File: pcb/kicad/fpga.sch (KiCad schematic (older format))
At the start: 1 part, among them U4 XC3S400-PQ208

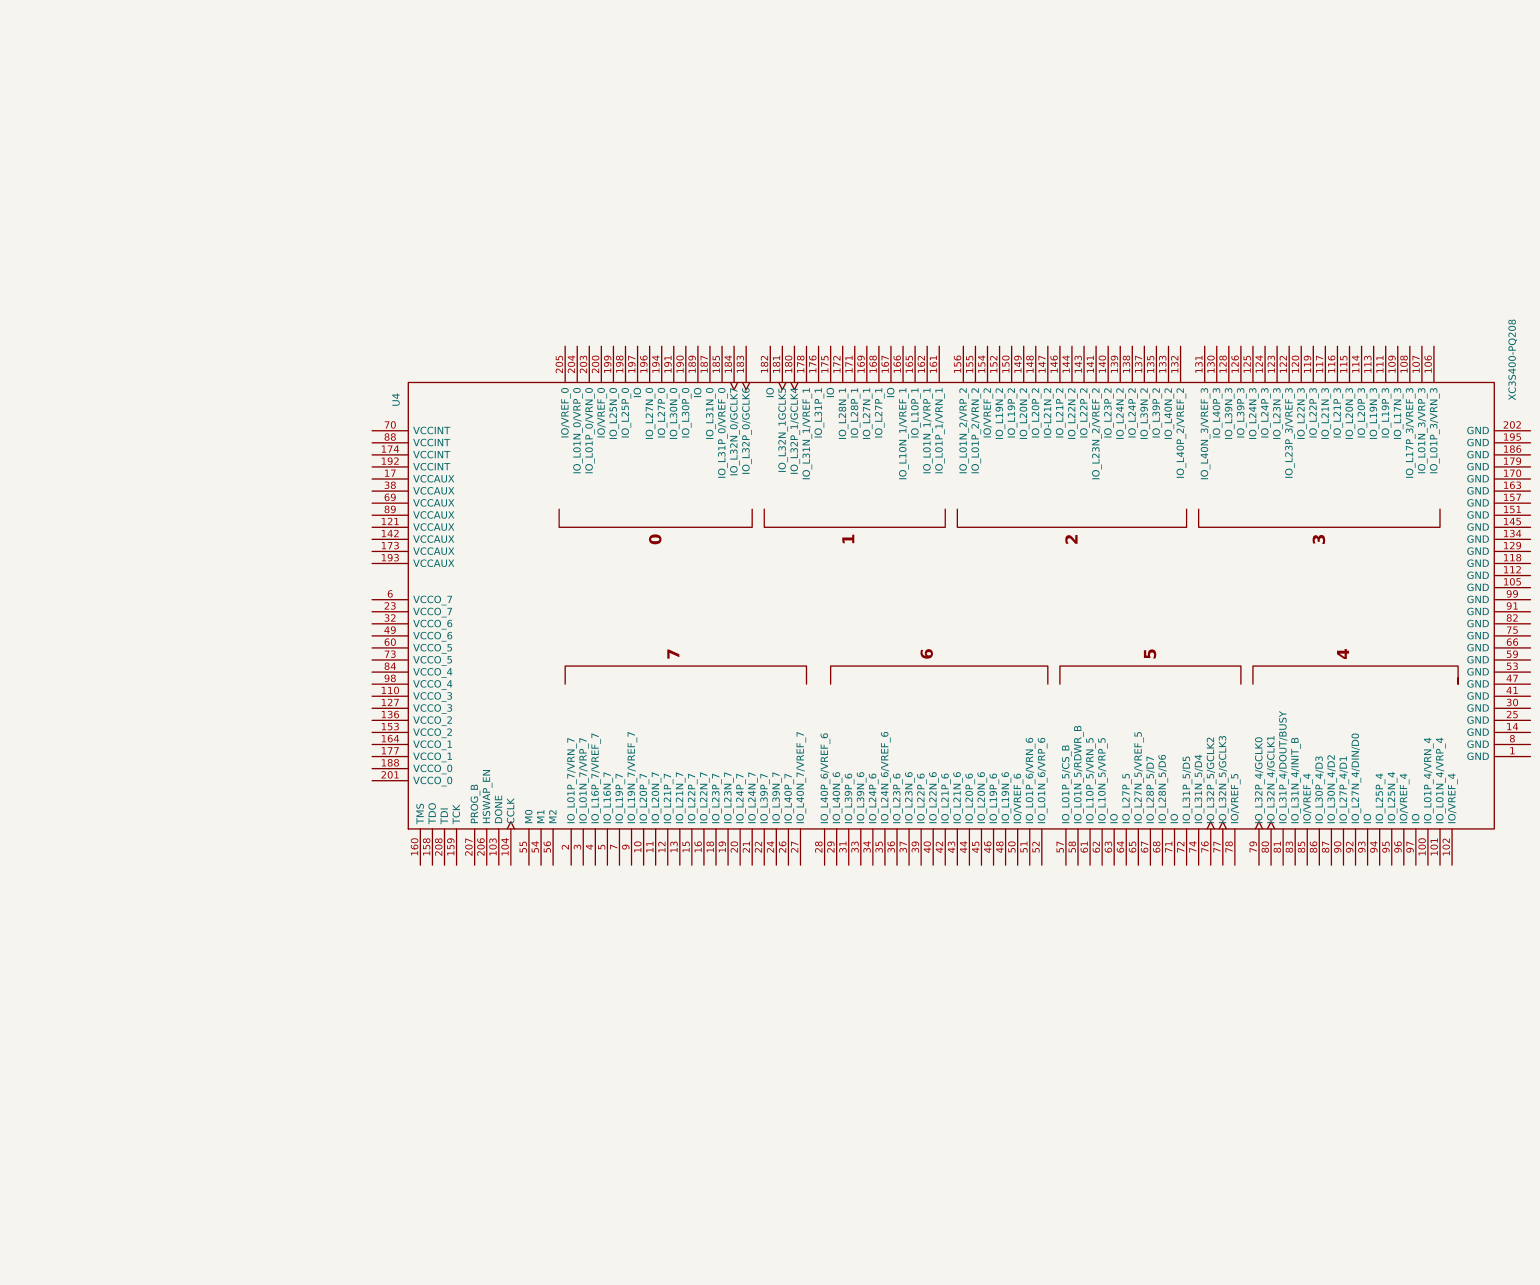
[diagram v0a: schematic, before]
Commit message: kicad wip
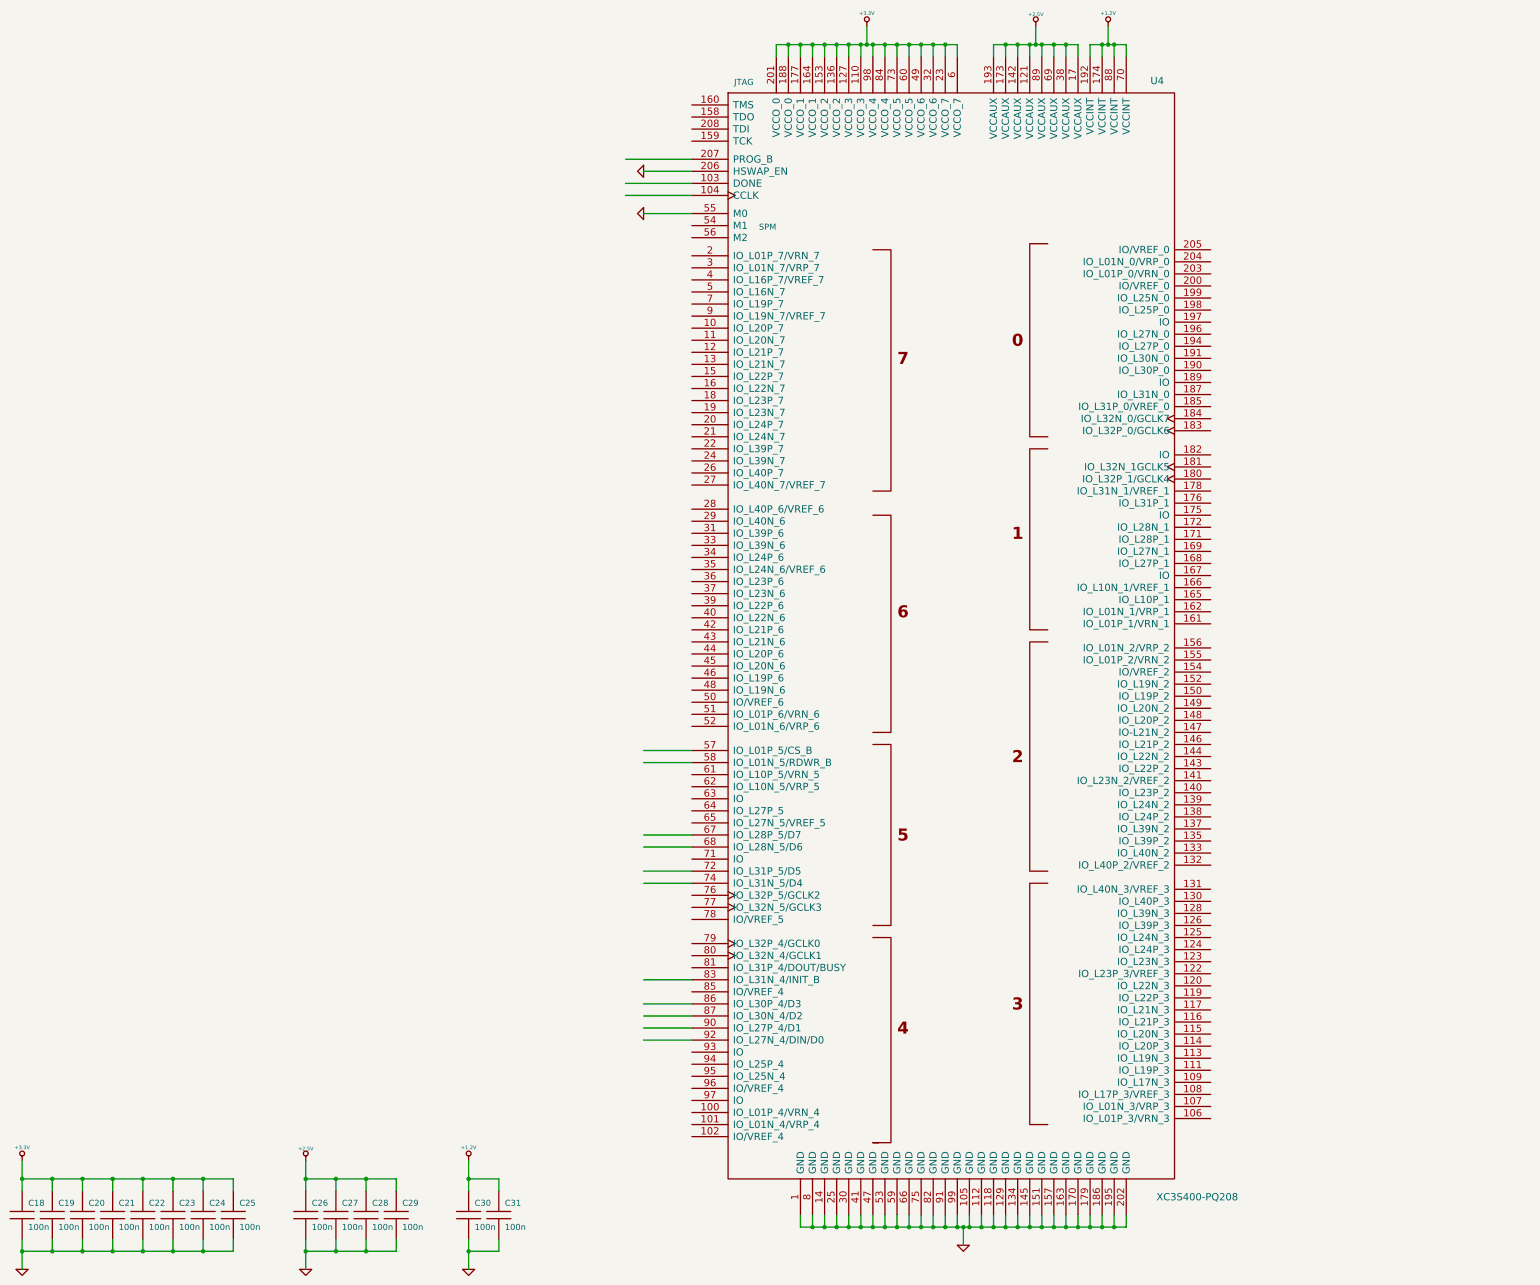
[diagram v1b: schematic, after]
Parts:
- added C18, C19, C20, C21, C22, C23, C24, C25, C26, C27, C28, C29, C30, C31: 100n, symbol C
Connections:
- net labels added: +1.2V, +2.5V, +3.3V, GND
- wire segments 0 -> 114
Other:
- note added: "JTAG"
- note added: "SPM"
- moved on the sheet: U4

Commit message: Schematics+PCB WIP
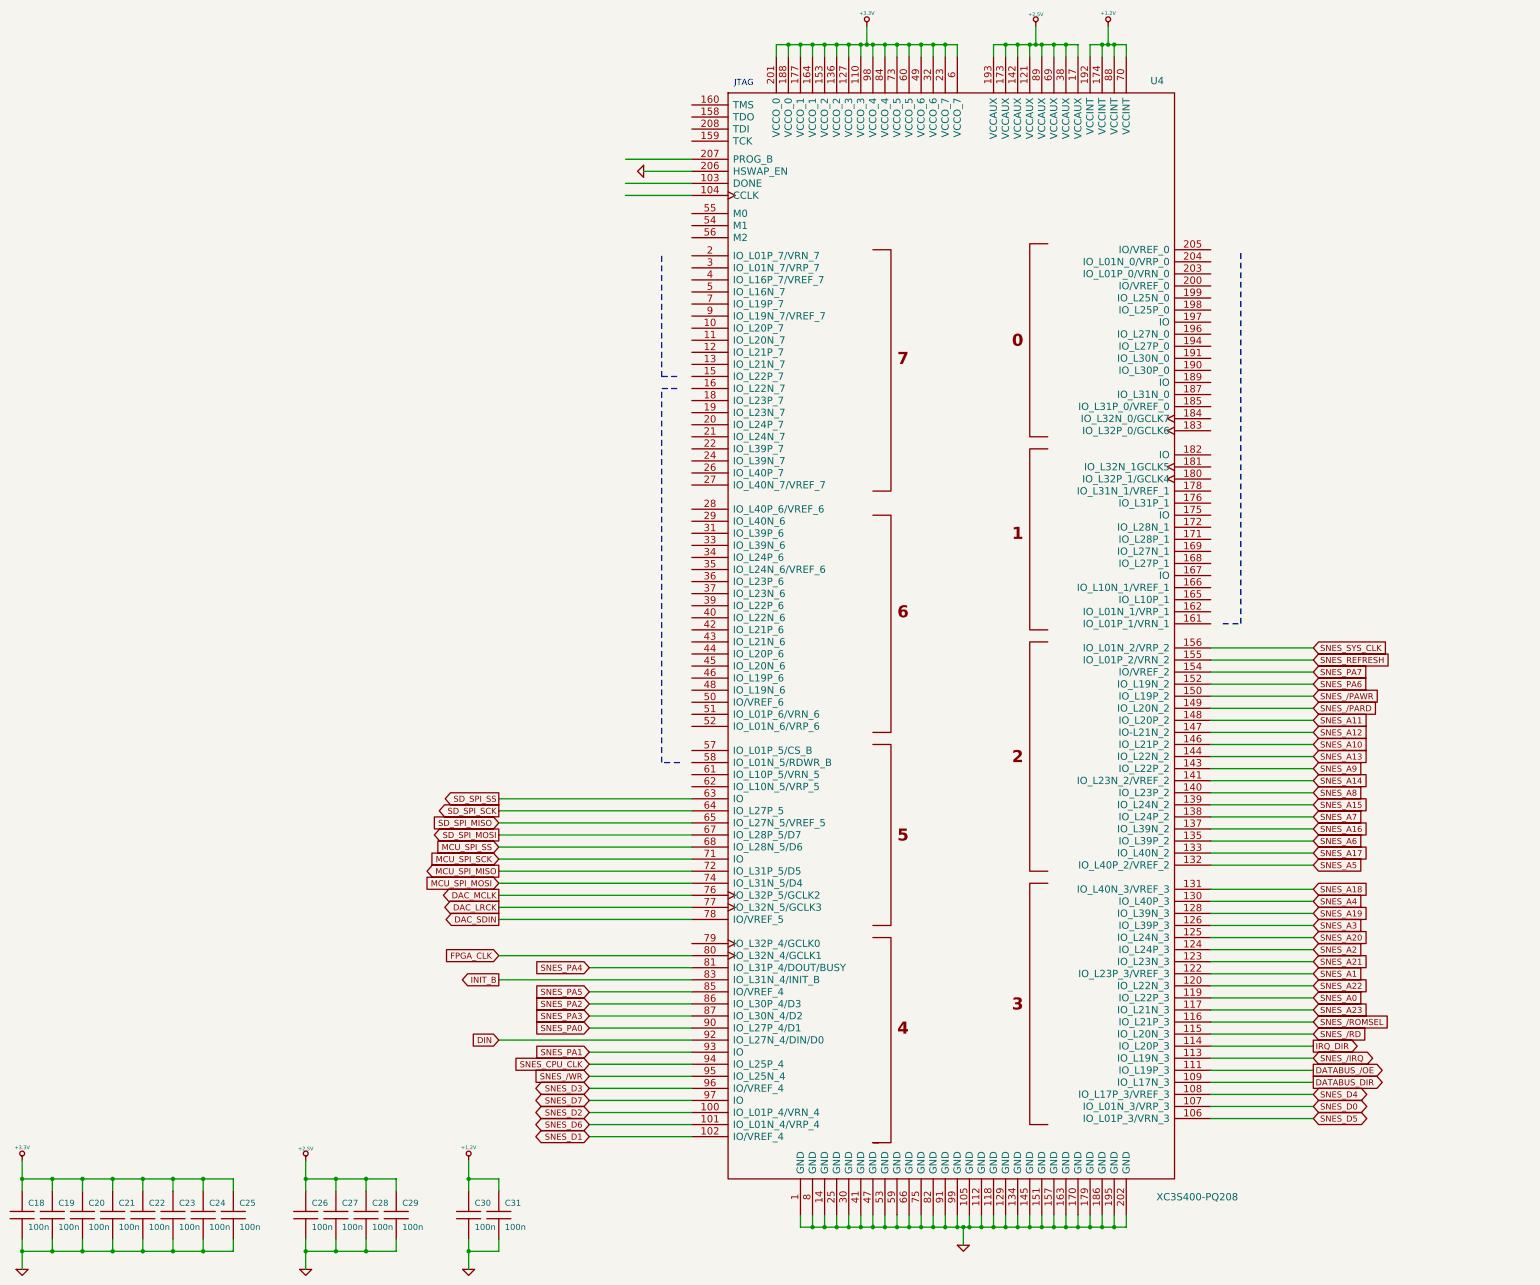
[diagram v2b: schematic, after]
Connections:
- net labels added: DAC_LRCK, DAC_MCLK, DAC_SDIN, DATABUS_/OE, DATABUS_DIR, DIN, FPGA_CLK, INIT_B, IRQ_DIR, MCU_SPI_MISO, MCU_SPI_MOSI, MCU_SPI_SCK, MCU_SPI_SS, SD_SPI_MISO, SD_SPI_MOSI, SD_SPI_SCK, SD_SPI_SS, SNES_/IRQ, SNES_/PARD, SNES_/PAWR, SNES_/RD, SNES_/ROMSEL, SNES_/WR, SNES_A0, SNES_A1, SNES_A10, SNES_A11, SNES_A12, SNES_A13, SNES_A14, SNES_A15, SNES_A16, SNES_A17, SNES_A18, SNES_A19, SNES_A2, SNES_A20, SNES_A21, SNES_A22, SNES_A23, SNES_A3, SNES_A4, SNES_A5, SNES_A6, SNES_A7, SNES_A8, SNES_A9, SNES_CPU_CLK, SNES_D0, SNES_D1, SNES_D2, SNES_D3, SNES_D4, SNES_D5, SNES_D6, SNES_D7, SNES_PA0, SNES_PA1, SNES_PA2, SNES_PA3, SNES_PA4, SNES_PA5, SNES_PA6, SNES_PA7, SNES_REFRESH, SNES_SYS_CLK
- wire segments 114 -> 168
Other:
- note removed: "SPM"
